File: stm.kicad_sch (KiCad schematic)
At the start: 32 parts, among them J1 USB_B_Micro, J2 Conn_01x04_Pin, J3 Conn_01x04_Pin, J4 Conn_01x04_Pin, SW1 SW_SPDT, U1 AMS1117-3.3, U2 STM32F103C8Tx, Y1 16MHz

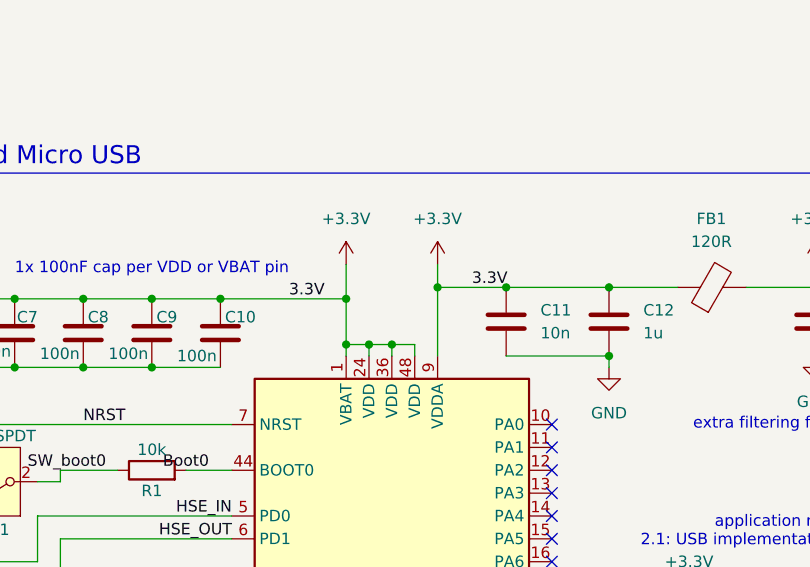
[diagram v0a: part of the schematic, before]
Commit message: done with proj
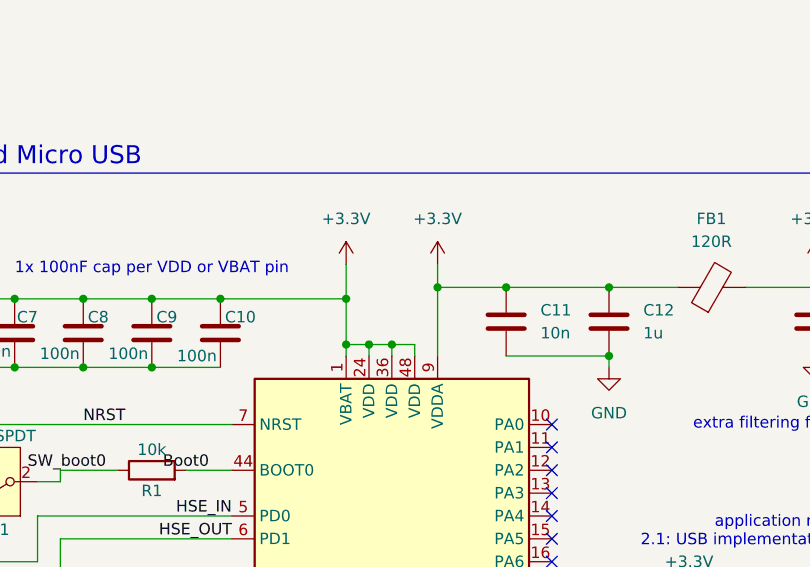
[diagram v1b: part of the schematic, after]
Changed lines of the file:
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@@
-		)
-	)
-	(label "3.3V"
-		(at 140.97 49.53 0)
-		(effects
-			(font
-				(size 1.27 1.27)
-			)
-			(justify left bottom)
 		)
 	)
@@
 		(effects
 			(font
-				(size 1.27 1.27)
-			)
-			(justify left bottom)
-		)
-	)
-	(label "3.3V"
-		(at 120.65 50.8 0)
-		(effects
-			(font
